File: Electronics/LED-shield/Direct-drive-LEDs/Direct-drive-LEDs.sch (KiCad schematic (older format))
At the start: 43 parts, among them J1 Conn_01x02_Male, Q1 MMBT3904, Q2 BS170F, Q3 MMBT3904, Q4 BS170F, Q5 MMBT3904, Q6 BS170F, Q7 MMBT3904, Q8 BS170F, U1 TLC2722, U2 TLC2722

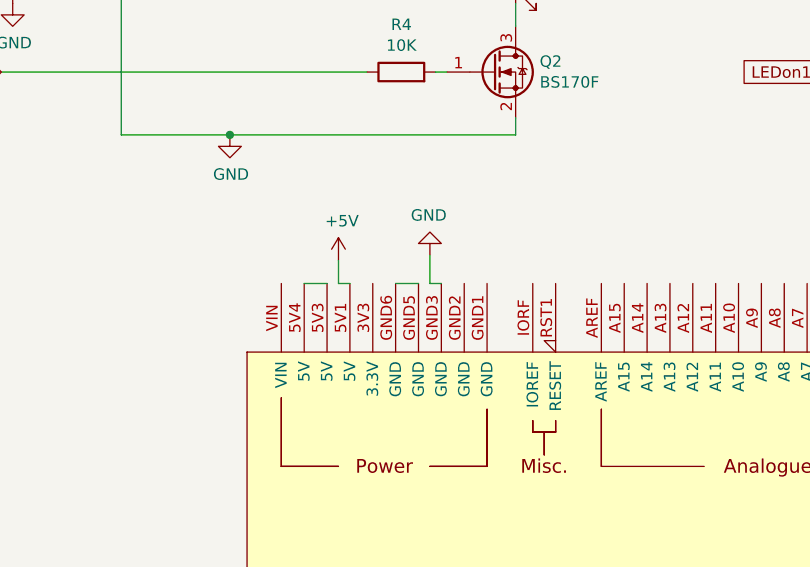
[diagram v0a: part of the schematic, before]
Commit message: PCB GERBERS.
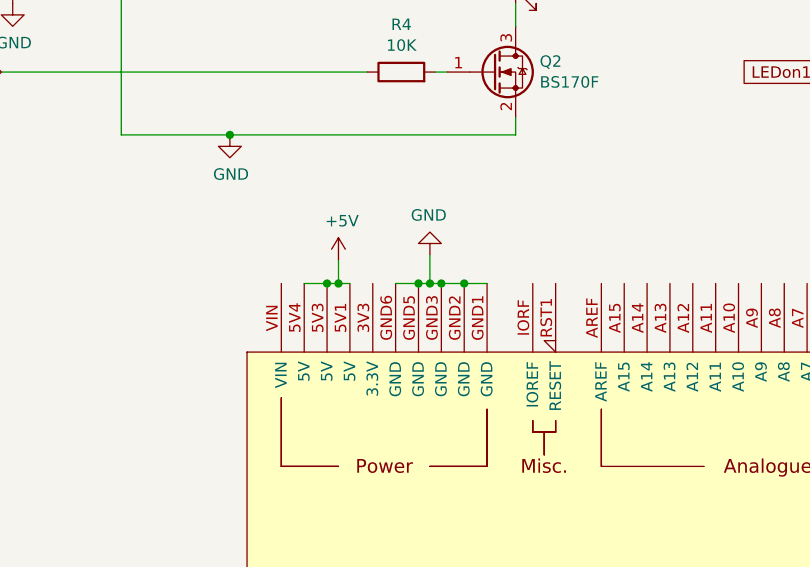
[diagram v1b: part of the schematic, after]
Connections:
- net +5V: now also XA1.5V3 (5V), XA1.5V4 (5V)
- net GND: now also XA1.GND1 (GND), XA1.GND2 (GND), XA1.GND5 (GND), XA1.GND6 (GND)
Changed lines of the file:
@@
 Connection ~ 2200 1400
 Connection ~ 9100 4250
+Wire Wire Line
+	2950 3725 3000 3725
+Connection ~ 2950 3725
+Connection ~ 3000 3725
+Wire Wire Line
+	3050 3725 3150 3725
+Connection ~ 3050 3725
+Wire Wire Line
+	3150 3725 3250 3725
+Connection ~ 3150 3725
+Wire Wire Line
+	2600 3725 2550 3725
+Connection ~ 2600 3725
+Connection ~ 2550 3725
 $EndSCHEMATC
